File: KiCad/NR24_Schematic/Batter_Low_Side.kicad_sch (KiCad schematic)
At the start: 9 parts

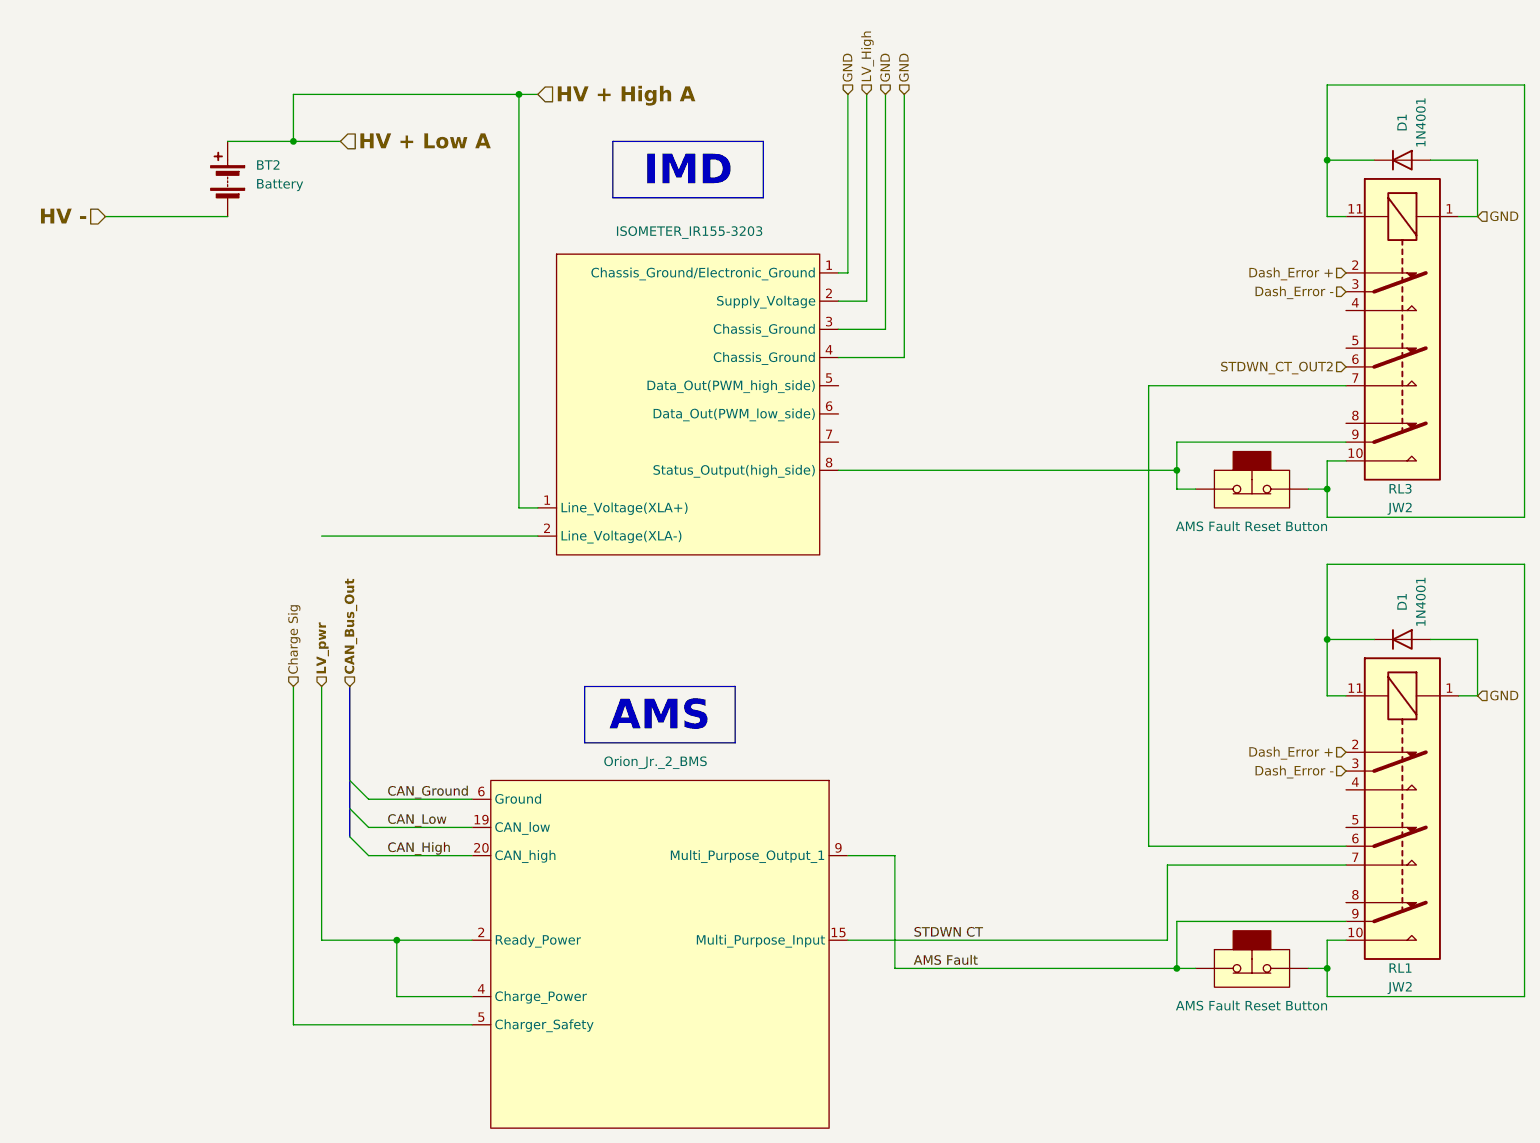
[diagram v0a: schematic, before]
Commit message: new sheet
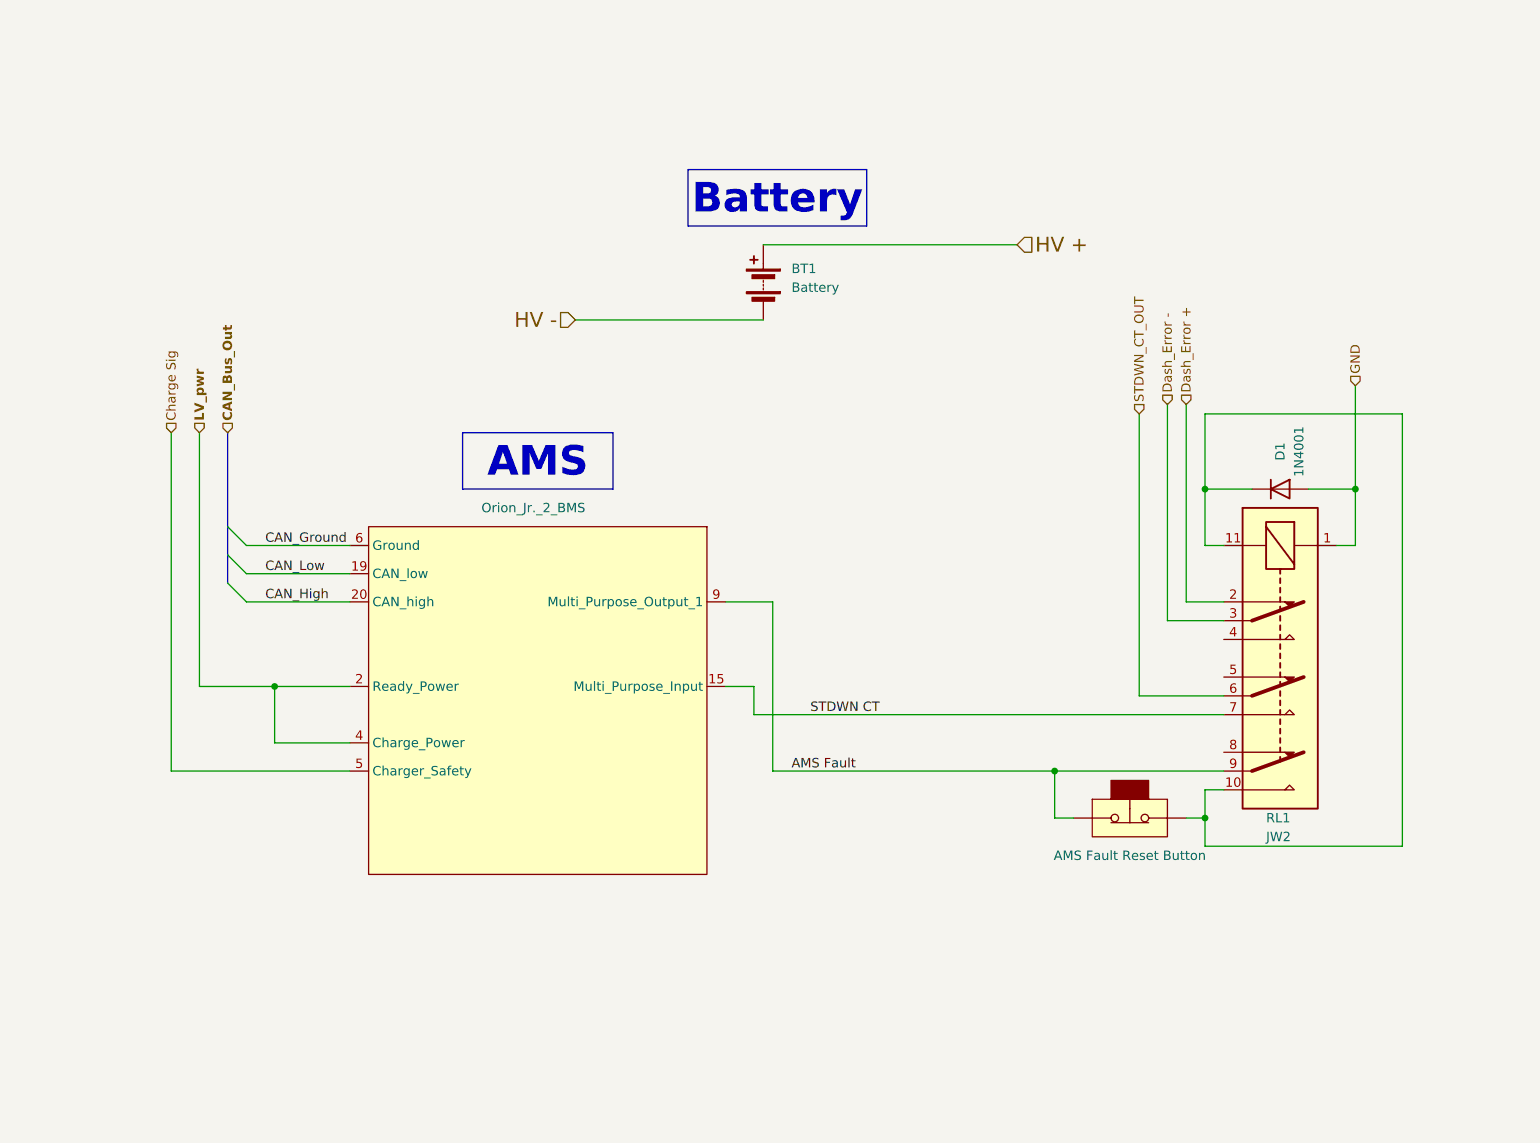
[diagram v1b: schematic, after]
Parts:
- removed BT2: Battery, symbol Device:Battery
- removed D1 (x2): 1N4001, Diode_THT:D_DO-41_SOD81_P10.16mm_Horizontal, symbol Diode:1N4001
- removed RL3: JW2, Relay_THT:Relay_DPDT_Panasonic_JW2, symbol Relay:JW2
- removed SW? (x2): AMS Fault Reset Button, symbol CamachosSymbols:Safety Switch
- removed U?: ISOMETER_IR155-3203, symbol CamachosSymbols:Sevcon_Gen4_Size6
- removed U?: Orion_Jr._2_BMS, symbol CamachosSymbols:Sevcon_Gen4_Size6
- added BT1: Battery, symbol Device:Battery
- added D1: 1N4001, Diode_THT:D_DO-41_SOD81_P10.16mm_Horizontal, symbol Diode:1N4001
- added SW?: AMS Fault Reset Button, symbol CamachosSymbols:Safety Switch
- added U?: Orion_Jr._2_BMS, symbol CamachosSymbols:Sevcon_Gen4_Size6
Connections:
- net AMS Fault: now also SW?.1 (A), U?.9 (Multi_Purpose_Output_1)
- net CAN_Ground: now also U?.6 (Ground)
- net CAN_High: now also U?.20 (CAN_high)
- net CAN_Low: now also U?.19 (CAN_low)
- net Charge Sig: now also U?.5 (Charger_Safety)
- net GND: now also D1.2 (A)
- net HV -: now also BT1.2 (-)
- net LV_pwr: now also U?.2 (Ready_Power), U?.4 (Charge_Power)
- net STDWN CT: now also U?.15 (Multi_Purpose_Input)
- net STDWN_CT_OUT: now reaches RL1.6
- net at RL1.10, RL1.11: now also D1.1 (K), SW?.2 (B)
- new net HV +: BT1.1 (+)
